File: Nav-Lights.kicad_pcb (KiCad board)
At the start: 4 copper layers, 41.6 x 10 mm, 28 parts, among them U1 LMC555CMMX, U2 TPS7B8133QWDRVRQ1, U3 LT8374RUFM-WPBF

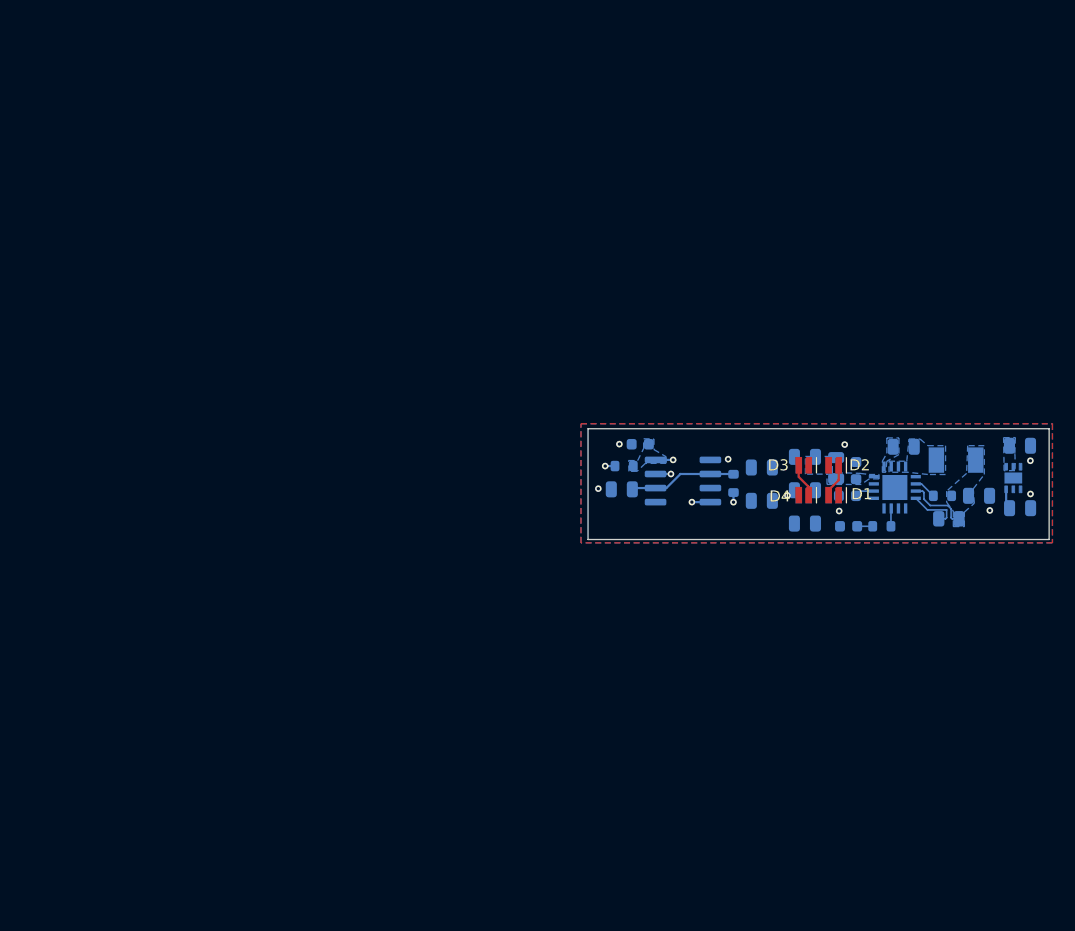
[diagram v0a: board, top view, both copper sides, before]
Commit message: Layout w/ connector
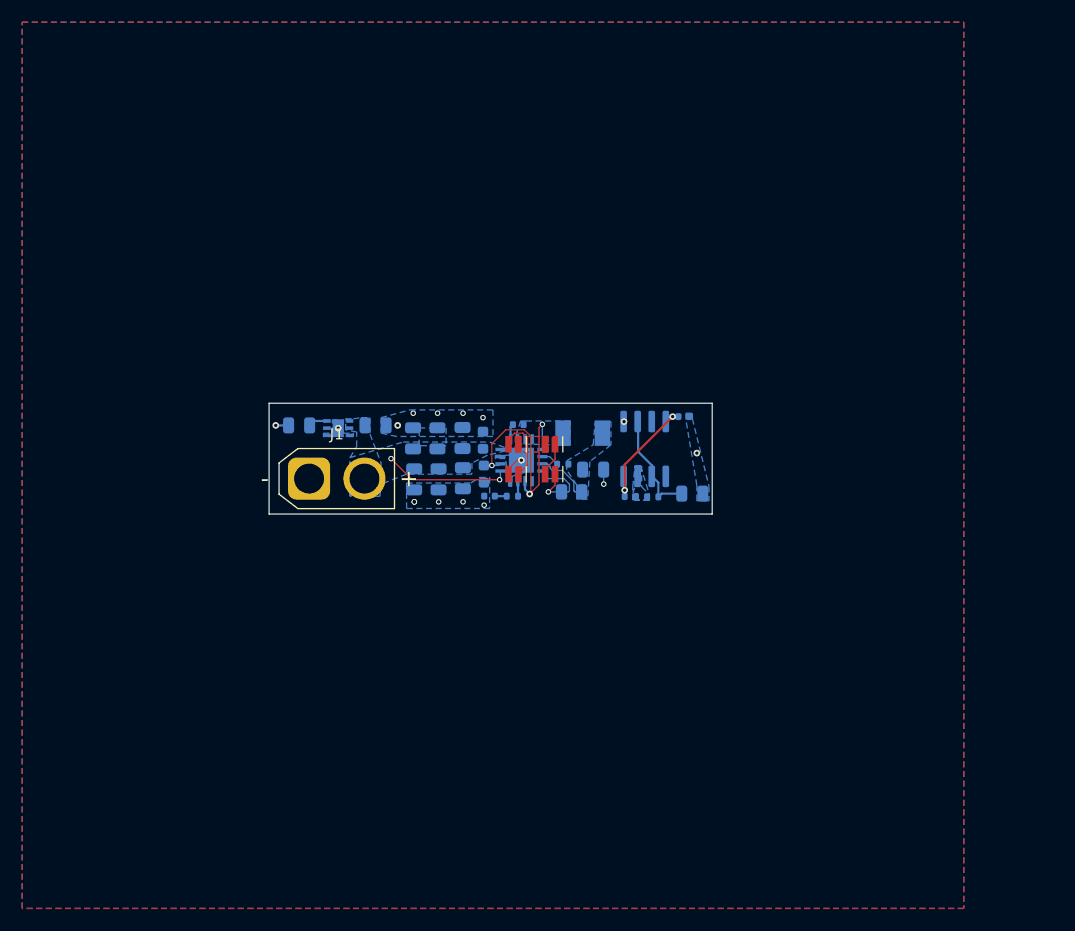
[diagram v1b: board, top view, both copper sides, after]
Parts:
- added J1: Conn_01x02_Pin, Connector_AMASS:AMASS_XT30U-M_1x02_P5.0mm_Vertical, F.Cu at (130.9, 96.2)
- C4, C7: footprint Capacitor_SMD:C_0603_1608Metric -> Capacitor_SMD:C_0402_1005Metric
- C9: footprint Capacitor_SMD:C_0805_2012Metric -> Capacitor_SMD:C_0402_1005Metric
- R1, R2, R3, R4: footprint Resistor_SMD:R_0603_1608Metric -> Resistor_SMD:R_0402_1005Metric
- moved C5 65.5 mm to (130.0, 91.4), turned to 180 degrees
- moved U2 61.1 mm to (133.5, 91.7), turned to 180 degrees
- moved C1 58.2 mm to (136.9, 91.4)
- moved C13 35.7 mm to (140.3, 92.6), turned to 90 degrees
- moved C14 35.5 mm to (140.4, 96.3), turned to -90 degrees
- moved C6 34.9 mm to (156.5, 95.4)
- moved C9 34.9 mm to (149.8, 91.3)
- moved R3 34.4 mm to (153.8, 94.9)
- moved R5 34.1 mm to (154.6, 97.4)
- moved C11 33.8 mm to (144.8, 92.5)
- moved U3 33.8 mm to (150.1, 94.5)
- moved L1 33.8 mm to (155.6, 92.1)
- moved C10 33.8 mm to (146.6, 92.7)
- moved R4 33.5 mm to (149.2, 97.8)
- moved C12 33.2 mm to (142.5, 92.6), turned to 90 degrees
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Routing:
- net GND: track 0.00 -> 69.6 mm, vias 1 -> 17
- net /Main/INTVCC: track 1.78 -> 23.8 mm, vias 0 -> 3
- net /Main/VIN: track 0.00 -> 11.4 mm, vias 0 -> 2
- net +3V3: track 5.31 -> 13.3 mm
- net Net-(U1-DIS): track 3.14 -> 0.00 mm, vias 3 -> 0
- net Net-(D3-K): track 3.07 -> 6.19 mm
- net /Main/ISN: track 4.67 -> 7.52 mm, vias 0 -> 1
- net Net-(U3-BST): track 0.00 -> 1.41 mm
- net /Main/ISP: track 5.75 -> 5.16 mm
- net (no net): vias 8 -> 0
- added copper zone on F.Cu, net Net-(D2-K)
- added copper zone on B.Cu, net Net-(U1-DIS)
- removed copper zone on B.Cu, net +3V3
- removed copper zone on B.Cu, net Net-(U3-BST)
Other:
- board size 41.6 x 10 mm -> 40 x 10 mm
